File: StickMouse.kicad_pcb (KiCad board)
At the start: 2 copper layers, 70 x 23 mm, 19 parts, among them J1 USB_B_Micro, J2 Joystick, J3 Debug, SW1 BTN_LEFT, SW2 BTN_RIGHT, U1 NJM78L33SU3, U2 STM32F042K6Tx

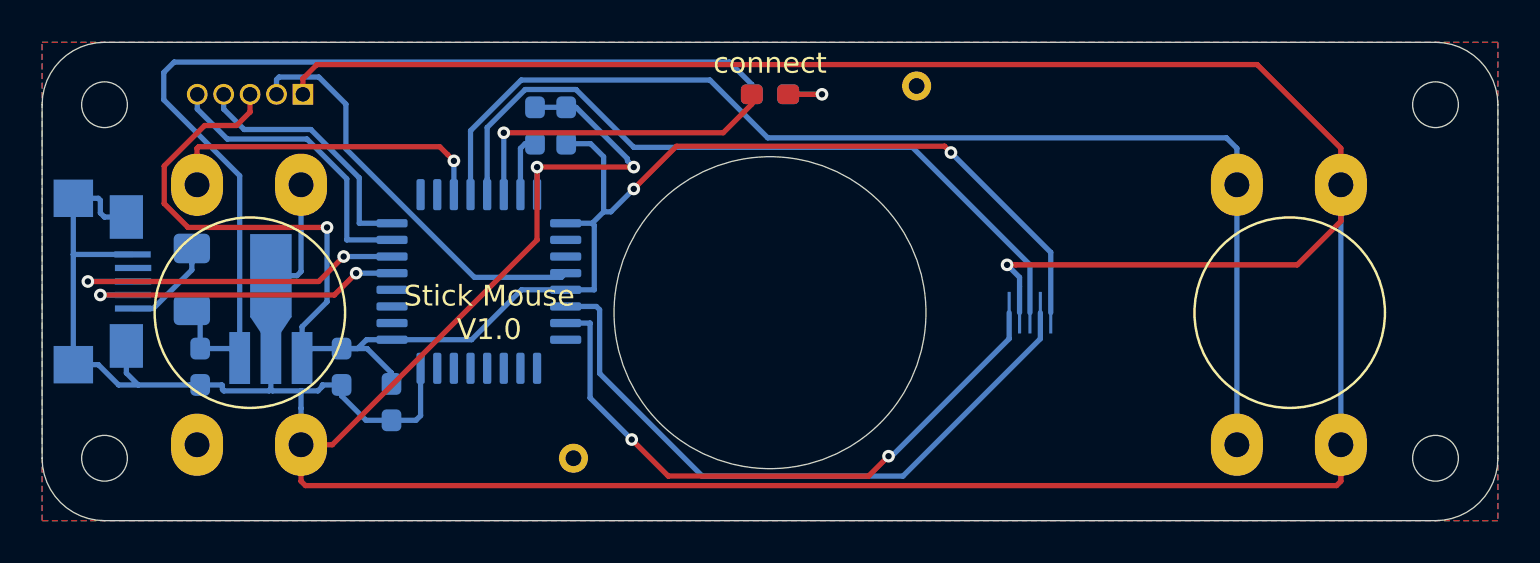
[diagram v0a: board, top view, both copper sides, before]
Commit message: 基板 V1.1
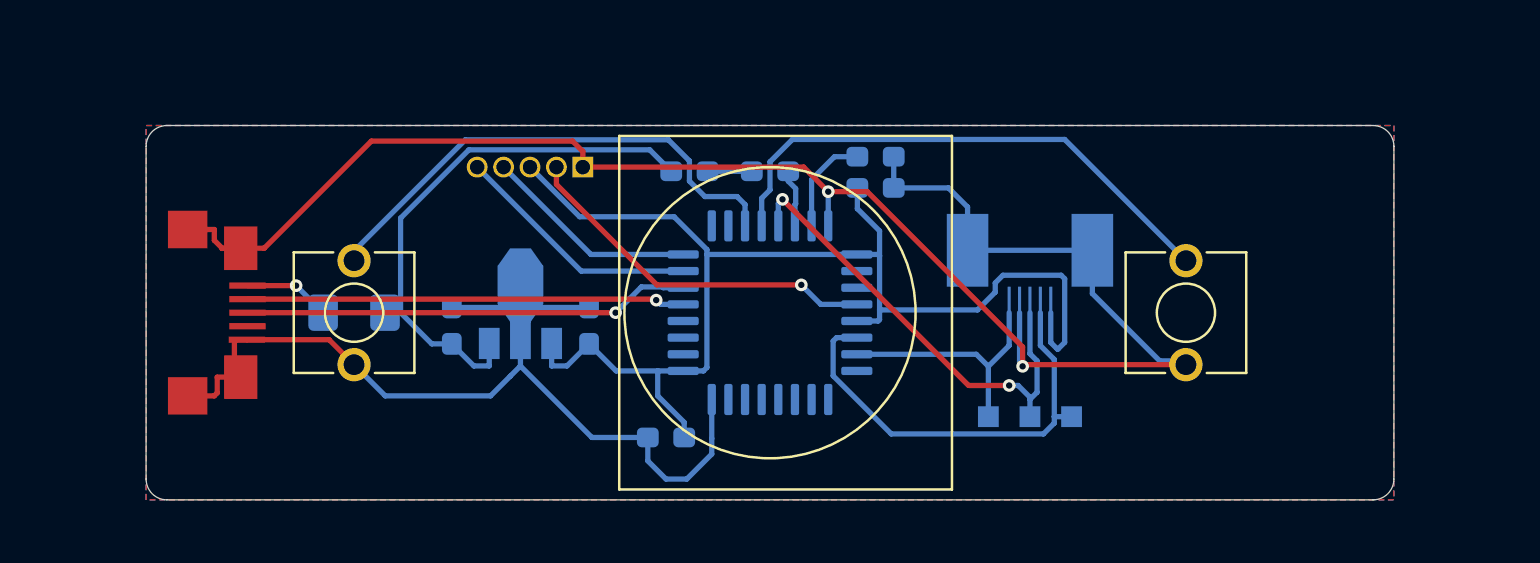
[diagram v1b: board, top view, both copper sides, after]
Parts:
- removed REF** (x4): MountingHole_2.2mm_M2, StickMouse:MountingHole_2.2mm_M2
- added TP1: BTN, TestPoint:TestPoint_Pad_1.0x1.0mm, B.Cu at (12.5, 5.00)
- added TP2: V, TestPoint:TestPoint_Pad_1.0x1.0mm, B.Cu at (14.5, 5.00)
- added TP3: H, TestPoint:TestPoint_Pad_1.0x1.0mm, B.Cu at (10.5, 5.00)
- D1: moved to B.Cu
- J1: moved to F.Cu
- SW1, SW2: footprint StickMouse:SW_PUSH-12mm_Custom -> StickMouse:Kailh_Mute_Switch
- U1: footprint Package_TO_SOT_SMD:SOT-89-3_Handsoldering -> Package_TO_SOT_SMD:SOT-89-3
- moved R1 16.4 mm to (5.08, -7.50), turned to 0 degrees
- moved C3 15.2 mm to (5.08, -6.00), turned to 0 degrees
- moved U2 14.1 mm to (0.00, 0.00)
- moved J3 13.9 mm to (-9.00, -7.00)
- moved C4 13.3 mm to (-5.00, 6.00), turned to 180 degrees
- moved C1 12.3 mm to (-15.3, 0.62), turned to 90 degrees
- moved C2 12.1 mm to (-8.70, 0.62), turned to 90 degrees
- moved U1 12.0 mm to (-12.0, 0.00)
- moved SW1 9.87 mm to (-20.0, 0.00), turned to 0 degrees
- moved F1 7.96 mm to (-20.0, 0.00), turned to 180 degrees
- moved SW2 6.81 mm to (20.0, 0.00), turned to 0 degrees
- moved J1 5.70 mm to (-28.0, 0.00), turned to 270 degrees
- moved R2 5.36 mm to (-3.88, -6.80)
- moved D1 3.70 mm to (0.00, -6.80), turned to 180 degrees
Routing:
- net GND: track 223.6 -> 130.0 mm, vias 3 -> 2
- net BTN_RIGHT: track 56.5 -> 26.1 mm
- net +5V: track 48.7 -> 26.5 mm
- net JOYSTICK_H: track 30.5 -> 12.0 mm, vias 2 -> 0
- net +3V3: track 79.6 -> 61.4 mm, vias 3 -> 0
- net JOYSTICK_BTN: track 35.9 -> 22.6 mm, vias 0 -> 2
- net LED_CONNECT: track 15.9 -> 2.84 mm, vias 1 -> 0
- net JOYSTICK_V: track 32.0 -> 21.3 mm
- net BTN_LEFT: track 16.0 -> 24.4 mm, vias 1 -> 0
- net USB_DM: track 16.0 -> 21.1 mm, vias 2 -> 1
- net USB_DP: track 17.3 -> 21.6 mm, vias 2 -> 1
- net SWDIO: track 14.4 -> 12.0 mm
- net NRST: track 20.0 -> 17.7 mm, vias 0 -> 1
- net SWCLK: track 12.4 -> 10.4 mm
- net Net-(R1-Pad1): track 3.02 -> 4.92 mm
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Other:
- board size 70 x 23 mm -> 60 x 18 mm
- board text added: "BTN"
- board text added: "H"
- board text added: "Micro USB"
- board text added: "Stick Mouse V1.1"
- board text added: "V"
- board text removed: "Stick Mouse V1.0"
